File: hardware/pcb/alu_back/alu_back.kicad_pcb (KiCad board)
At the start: 2 copper layers, 130.8 x 127.6 mm, 12 parts, among them J1 SYNC, J2 BUS, J3 FLAGS, U1 Register A, U2 Register B, U3 Register C, U4 Register D, U5 Add/Sub, U6 And/Or, U7 Xor/Not, U8 Shift, U9 Flags

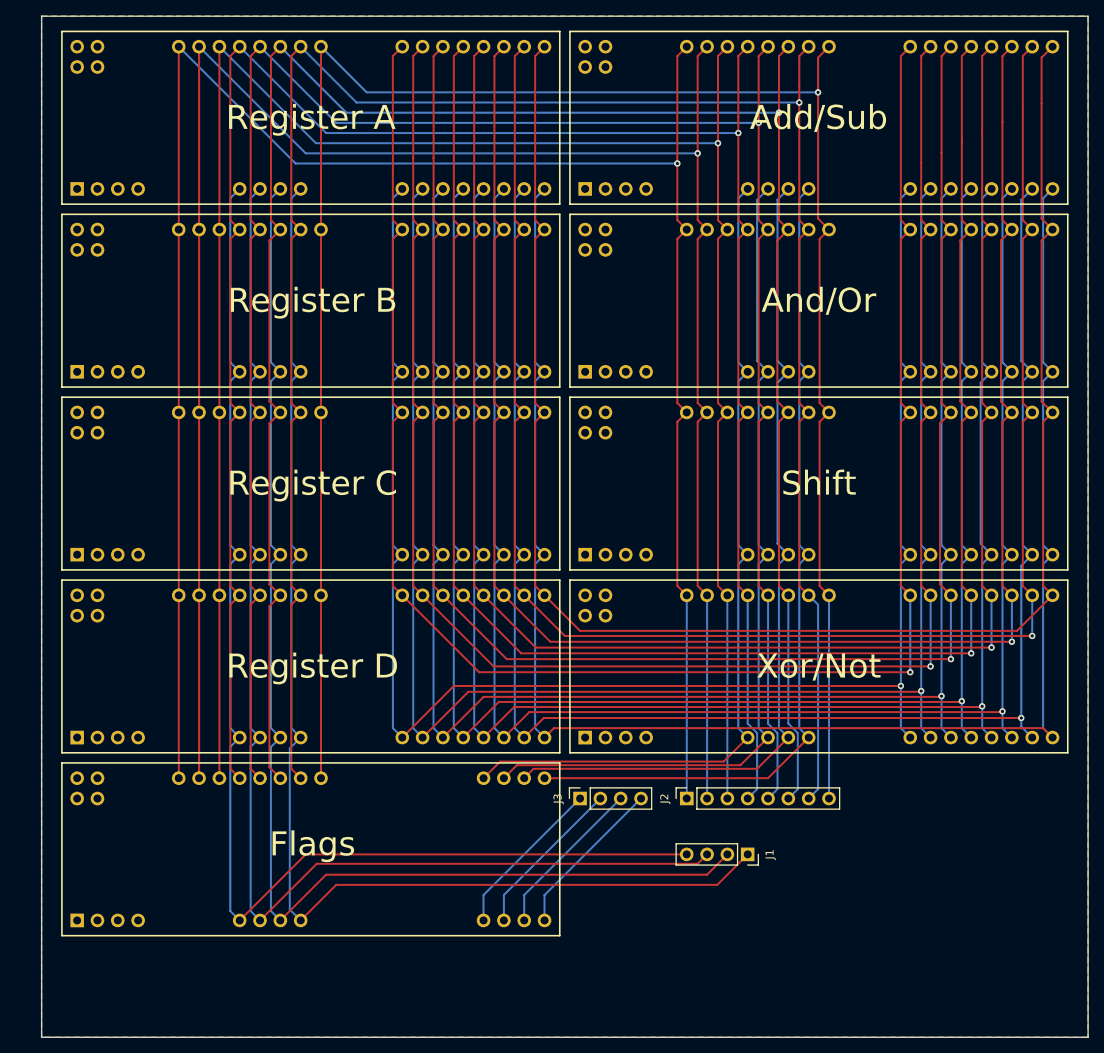
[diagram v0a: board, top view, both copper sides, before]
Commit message: ALU backplane board
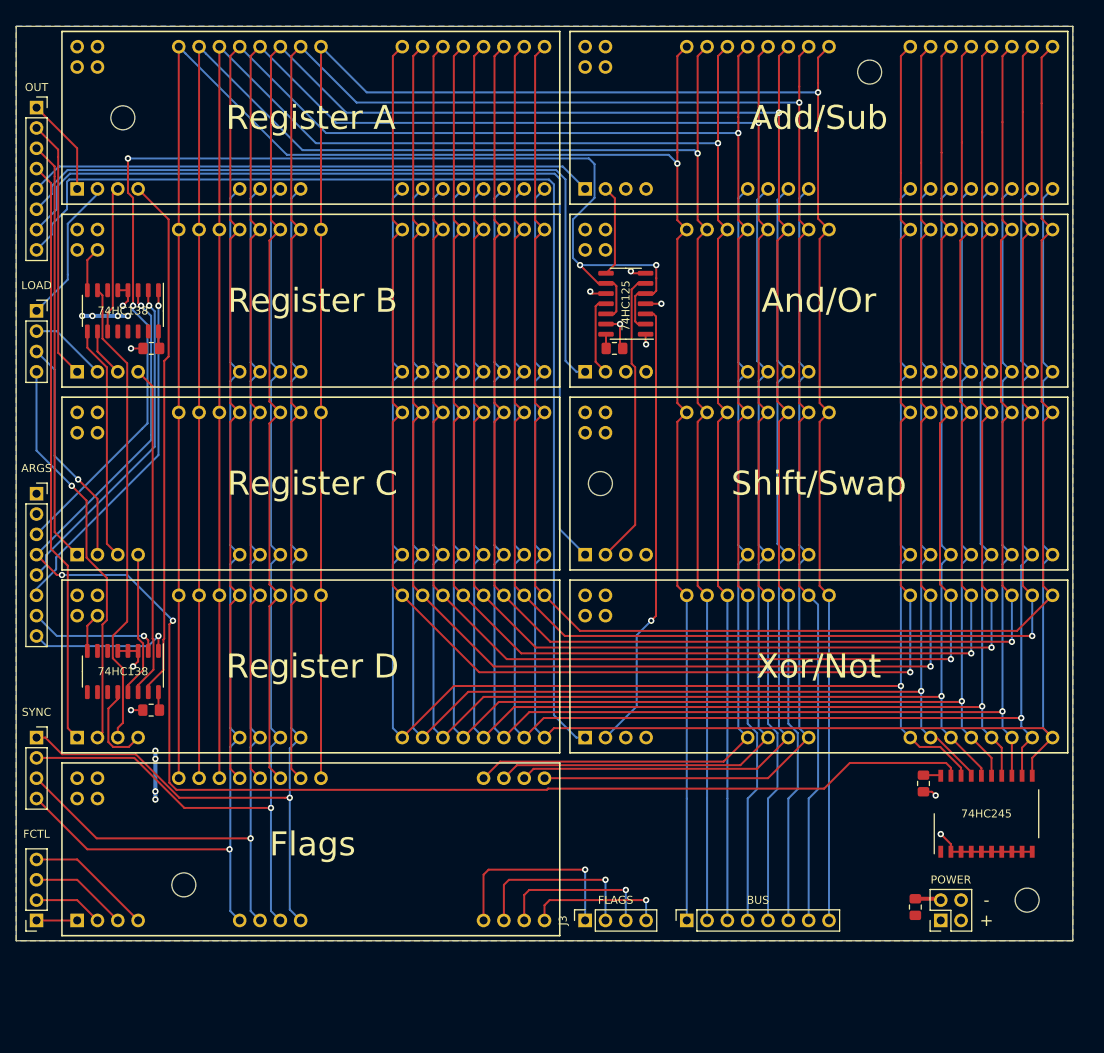
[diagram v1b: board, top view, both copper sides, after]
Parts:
- added C1: 10uF, Capacitor_SMD:C_0805_2012Metric_Pad1.18x1.45mm_HandSolder, F.Cu at (134.6, 134.9)
- added C2: 100nF, Capacitor_SMD:C_0805_2012Metric_Pad1.18x1.45mm_HandSolder, F.Cu at (39.1, 110.2)
- added C3: 100nF, Capacitor_SMD:C_0805_2012Metric_Pad1.18x1.45mm_HandSolder, F.Cu at (39.1, 65.0)
- added C4: 100nF, Capacitor_SMD:C_0805_2012Metric_Pad1.18x1.45mm_HandSolder, F.Cu at (97.0, 65.0)
- added C5: 100nF, Capacitor_SMD:C_0805_2012Metric_Pad1.18x1.45mm_HandSolder, F.Cu at (135.6, 119.4)
- added H1: MountingHole, MountingHole:MountingHole_3mm, F.Cu at (35.6, 36.2)
- added H2: MountingHole, MountingHole:MountingHole_3mm, F.Cu at (43.2, 132.1)
- added H3: MountingHole, MountingHole:MountingHole_3mm, F.Cu at (148.6, 134.0)
- added H4: MountingHole, MountingHole:MountingHole_3mm, F.Cu at (128.9, 30.5)
- added H5: MountingHole, MountingHole:MountingHole_3mm, F.Cu at (95.2, 81.9)
- added J4: OUT, Connector_PinSocket_2.54mm:PinSocket_1x08_P2.54mm_Vertical, F.Cu at (24.8, 34.9)
- added J5: FCTL, Connector_PinSocket_2.54mm:PinSocket_1x04_P2.54mm_Vertical, F.Cu at (24.8, 136.5)
- added J6: LOAD, Connector_PinSocket_2.54mm:PinSocket_1x04_P2.54mm_Vertical, F.Cu at (24.8, 60.3)
- added J7: ARGS, Connector_PinSocket_2.54mm:PinSocket_1x08_P2.54mm_Vertical, F.Cu at (24.8, 83.2)
- added J8: POWER, Connector_PinSocket_2.54mm:PinSocket_2x02_P2.54mm_Vertical, F.Cu at (137.8, 136.5)
- added U10: 74HC125, Package_SO:SO-14_3.9x8.65mm_P1.27mm, F.Cu at (98.4, 59.4)
- added U11: 74HC245, Package_SO:SO-20_12.8x7.5mm_P1.27mm, F.Cu at (143.5, 123.2)
- added U12: 74HC138, Package_SO:SO-16_3.9x9.9mm_P1.27mm, F.Cu at (35.6, 105.4)
- added U13: 74HC138, Package_SO:SO-16_3.9x9.9mm_P1.27mm, F.Cu at (35.6, 60.3)
- U8: value Shift -> Shift/Swap
- moved J1 90.1 mm to (24.8, 113.7), turned to 0 degrees
- moved J3 15.3 mm to (93.3, 136.5)
- moved J2 15.2 mm to (106.0, 136.5)
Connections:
- U1 pad 1: Net-(U1-Pad1) -> OUT_A
- U1 pad 2: Net-(U1-Pad2) -> LOAD_A
- U1 pad 3: Net-(U1-Pad3) -> ARG_AA
- U1 pad 4: Net-(U1-Pad4) -> ARG_AB
- U2 pad 1: Net-(U2-Pad1) -> OUT_B
- U2 pad 2: Net-(U2-Pad2) -> LOAD_B
- U2 pad 3: Net-(U2-Pad3) -> ARG_BA
- U2 pad 4: Net-(U2-Pad4) -> ARG_BB
- U3 pad 1: Net-(U3-Pad1) -> OUT_C
- U3 pad 2: Net-(U3-Pad2) -> LOAD_C
- U3 pad 3: Net-(U3-Pad3) -> ARG_CA
- U3 pad 4: Net-(U3-Pad4) -> ARG_CB
- U4 pad 1: Net-(U4-Pad1) -> OUT_D
- U4 pad 2: Net-(U4-Pad2) -> LOAD_D
- U4 pad 3: Net-(U4-Pad3) -> ARG_DA
- U4 pad 4: Net-(U4-Pad4) -> ARG_DB
- U5 pad 1: Net-(U5-Pad1) -> OUT_AS
- U5 pad 2: Net-(U5-Pad2) -> ALT_AS
- U6 pad 1: Net-(U6-Pad1) -> OUT_AO
- U6 pad 2: Net-(U6-Pad2) -> ALT_AO
- U7 pad 1: Net-(U7-Pad1) -> OUT_XN
- U7 pad 2: Net-(U7-Pad2) -> ALT_XN
- U8 pad 1: Net-(U8-Pad1) -> OUT_S
- U8 pad 2: Net-(U8-Pad2) -> ALT_S
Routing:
- net ARG_B2: track 0.00 -> 181.3 mm, vias 0 -> 3
- net ALT: track 0.00 -> 156.9 mm, vias 0 -> 4
- net OUT_XN: track 0.00 -> 142.7 mm
- net OUT_S: track 0.00 -> 118.5 mm
- net OUT_AO: track 0.00 -> 94.9 mm
- net OUT_D: track 0.00 -> 73.2 mm
- net OUT_AS: track 0.00 -> 70.9 mm
- net ARG_AB: track 0.00 -> 65.5 mm
- net ARG_DA: track 0.00 -> 59.0 mm
- net ALT_XN: track 0.00 -> 56.7 mm, vias 0 -> 1
- net OUT_C: track 0.00 -> 52.9 mm
- net GND: track 0.00 -> 51.8 mm, vias 0 -> 11
- net LOAD_D: track 0.00 -> 49.8 mm, vias 0 -> 1
- net ARG_B0: track 0.00 -> 44.4 mm, vias 0 -> 1
- net ARG_B1: track 0.00 -> 42.0 mm, vias 0 -> 1
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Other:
- board size 130.8 x 127.6 mm -> 132.1 x 114.3 mm
- board text added: "+"
- board text added: "-"
